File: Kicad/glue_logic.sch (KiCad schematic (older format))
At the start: 17 parts, among them U12 SN74LS273, U13 DM74AS74M, U14 DM74AS74M, U15 74AS04, U16 DM74S05M, U17 74F151A, U18 DM74AS74M, U19 74F151A, U37 DM74AS74M, U5 DM74S05M, U51 DM74AS74M, U7 DM74AS74M

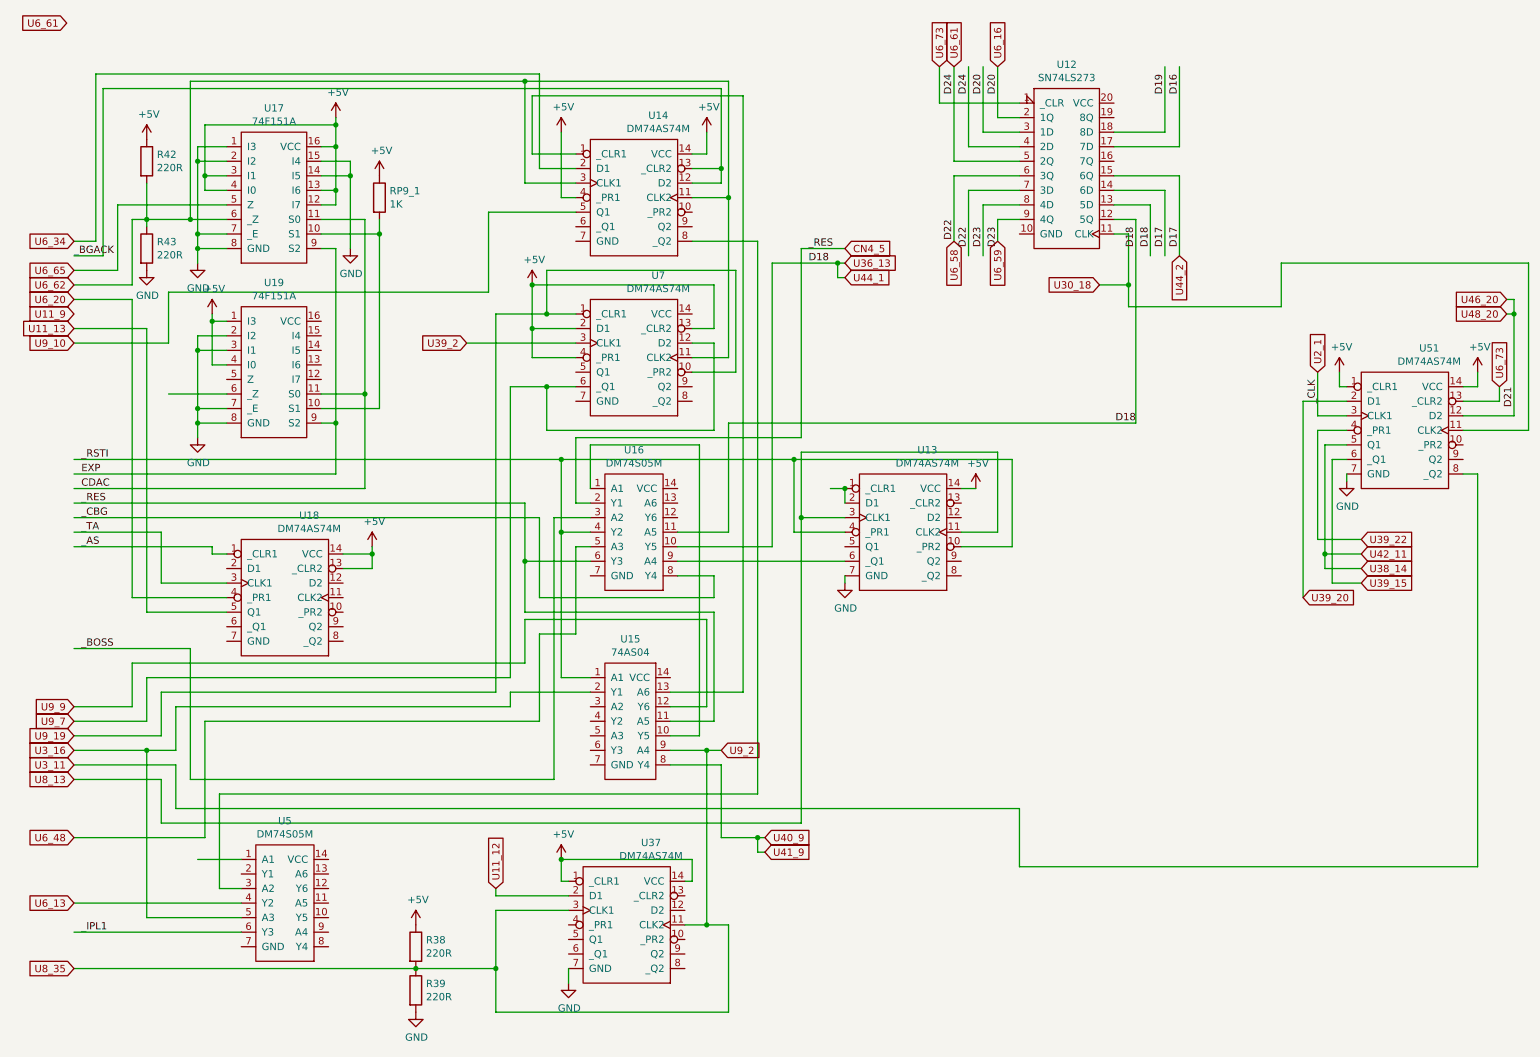
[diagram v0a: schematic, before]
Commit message: amother day, another tracks..
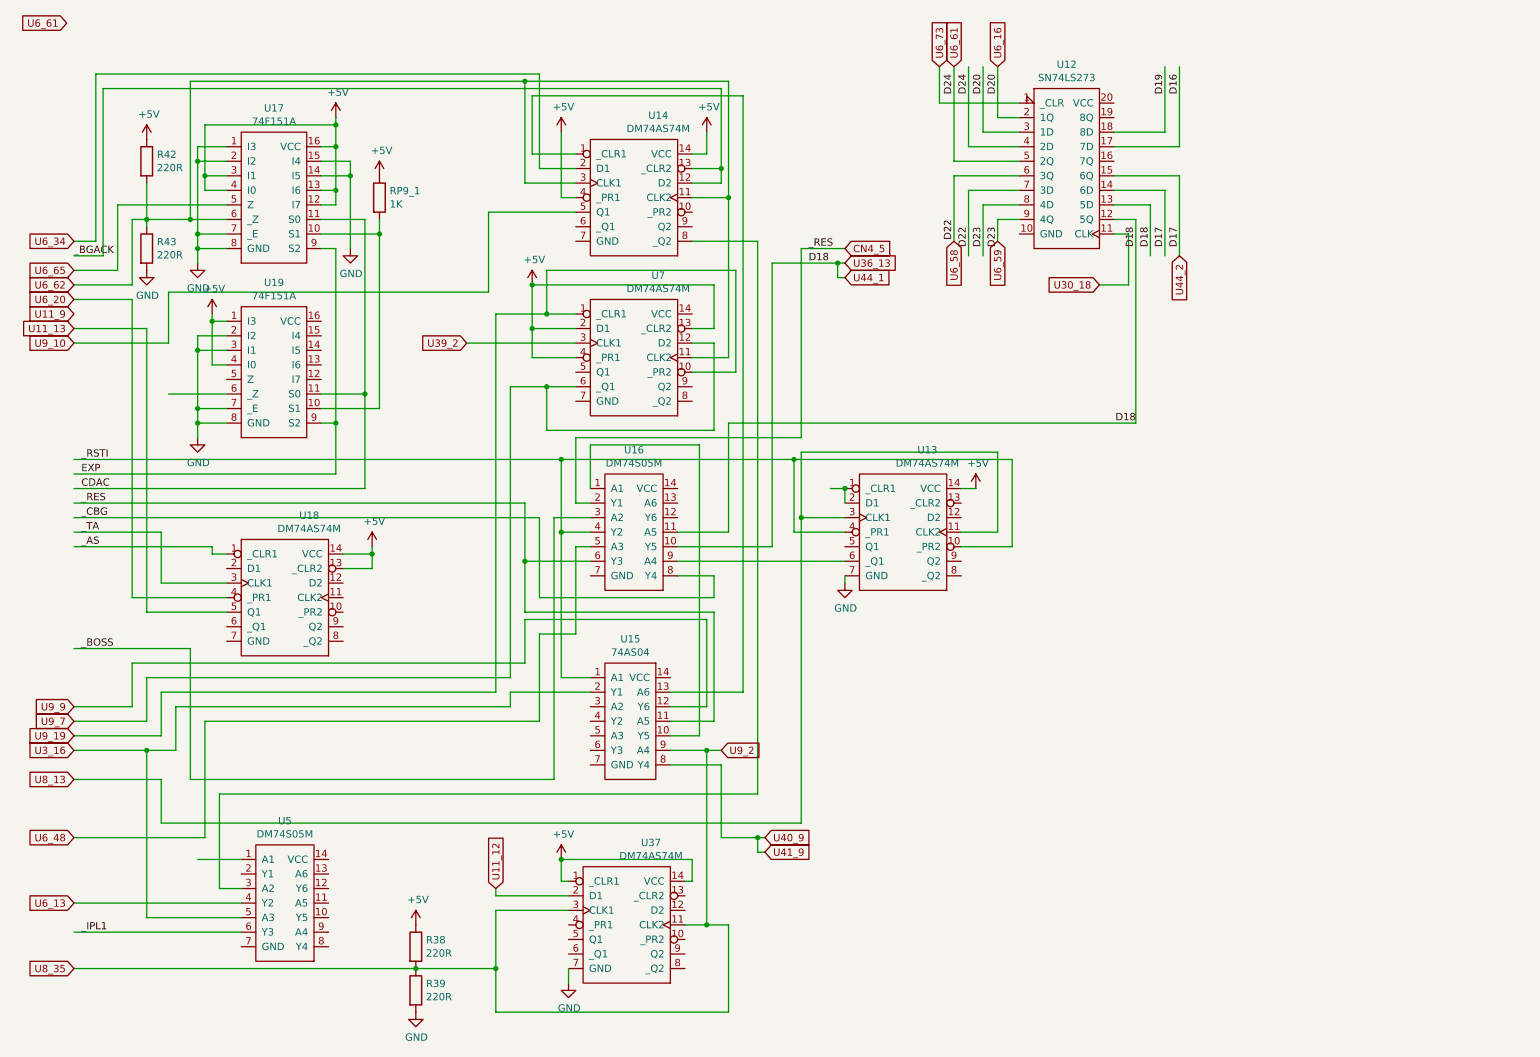
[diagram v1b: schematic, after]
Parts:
- removed U51: DM74AS74M, symbol New_Library_0:DM74AS74M
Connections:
- net labels removed: D21, U2_1, U38_14, U39_15, U39_20, U39_22, U3_11, U42_11, U46_20, U48_20, _CLK
- wire segments 329 -> 289
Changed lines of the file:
@@
 Wire Wire Line
 	4100 5250 4650 5250
-Text GLabel 1100 5750 0    50   Input ~ 0
-U3_11
-Wire Wire Line
-	1800 6050 1800 5750
-Wire Wire Line
-	1800 5750 1100 5750
 Text GLabel 1100 5850 0    50   Input ~ 0
 U8_13
@@
 Wire Wire Line
 	2250 6700 1100 6700
-Wire Wire Line
-	2100 5950 2100 6600
-Wire Wire Line
-	2100 6600 2250 6600
-Wire Wire Line
-	2100 5950 5800 5950
 Wire Wire Line
 	5800 5950 5800 2150
@@
 Wire Wire Line
 	3150 4300 3150 4250
-Wire Wire Line
-	10750 3150 10650 3150
-Wire Wire Line
-	10750 3050 10750 3150
-$Comp
-L power:+5V #PWR?
-U 1 1 5DC2CB2C
-P 10750 3050
-F 0 "#PWR?" H 10750 2900 50  0001 C CNN
-F 1 "+5V" H 10765 3223 50  0000 C CNN
-F 2 "" H 10750 3050 50  0001 C CNN
-F 3 "" H 10750 3050 50  0001 C CNN
-	1    10750 3050
-	1    0    0    -1
-$EndComp
-Wire Wire Line
-	9850 3800 9850 3750
-$Comp
-L power:GND #PWR?
-U 1 1 5DC0BA94
-P 9850 3800
-F 0 "#PWR?" H 9850 3550 50  0001 C CNN
-F 1 "GND" H 9855 3627 50  0000 C CNN
-F 2 "" H 9850 3800 50  0001 C CNN
-F 3 "" H 9850 3800 50  0001 C CNN
-	1    9850 3800
-	1    0    0    -1
-$EndComp
-Text GLabel 9550 4600 2    50   Input ~ 0
-U39_20
-Wire Wire Line
-	9850 3250 9550 3250
-Wire Wire Line
-	9750 4500 9950 4500
-Wire Wire Line
-	9750 3650 9750 4500
-Wire Wire Line
-	9850 3650 9750 3650
-Text GLabel 9950 4500 2    50   Input ~ 0
-U39_15
-Connection ~ 9700 4300
-Wire Wire Line
-	9700 4400 9700 4300
-Wire Wire Line
-	9950 4400 9700 4400
-Wire Wire Line
-	9700 4300 9950 4300
-Wire Wire Line
-	9700 3550 9700 4300
-Wire Wire Line
-	9850 3550 9700 3550
-Text GLabel 9950 4400 2    50   Input ~ 0
-U38_14
-Text GLabel 9950 4300 2    50   Input ~ 0
-U42_11
-Wire Wire Line
-	9650 4200 9950 4200
-Wire Wire Line
-	9650 3450 9650 4200
-Wire Wire Line
-	9850 3450 9650 3450
-Text GLabel 9950 4200 2    50   Input ~ 0
-U39_22
 Text GLabel 5850 6350 2    50   Input ~ 0
 U41_9
@@
 U40_9
 Wire Wire Line
-	9800 3150 9850 3150
-Wire Wire Line
-	9800 3050 9800 3150
-$Comp
-L power:+5V #PWR?
-U 1 1 5D8F16EA
-P 9800 3050
-F 0 "#PWR?" H 9800 2900 50  0001 C CNN
-F 1 "+5V" H 9815 3223 50  0000 C CNN
-F 2 "" H 9800 3050 50  0001 C CNN
-F 3 "" H 9800 3050 50  0001 C CNN
-	1    9800 3050
-	1    0    0    -1
-$EndComp
-$Comp
-L New_Library_0:DM74AS74M U51
-U 1 1 5DC69CD6
-P 10250 3450
-F 0 "U51" H 10417 4015 50  0000 C CNN
-F 1 "DM74AS74M" H 10417 3924 50  0000 C CNN
-F 2 "" H 10250 3450 50  0001 C CNN
-F 3 "" H 10250 3450 50  0001 C CNN
-	1    10250 3450
-	1    0    0    -1
-$EndComp
-Wire Wire Line
-	9550 3250 9550 4600
-Wire Wire Line
-	7600 6050 7600 6450
-Wire Wire Line
-	10750 6450 10750 3750
-Wire Wire Line
-	10750 3750 10650 3750
-Wire Wire Line
-	1800 6050 7600 6050
-Wire Wire Line
-	7600 6450 10750 6450
-Wire Wire Line
-	11100 2300 9400 2300
-Wire Wire Line
 	8350 2100 8350 2450
 Wire Wire Line
 	8150 2450 8350 2450
-Text GLabel 10900 3150 1    50   Input ~ 0
-U6_73
-Wire Wire Line
-	10900 3150 10900 3250
-Wire Wire Line
-	10650 3250 10900 3250
-Wire Wire Line
-	9850 3350 9650 3350
-Wire Wire Line
-	9650 3350 9650 3050
-Text GLabel 9650 3050 1    50   Input ~ 0
-U2_1
-Text Label 9650 3100 3    50   ~ 0
-_CLK
-Wire Wire Line
-	10650 3350 11000 3350
-Text Label 11000 3150 3    50   ~ 0
-D21
-Text GLabel 10950 2650 0    50   Input ~ 0
-U48_20
-Text GLabel 10950 2550 0    50   Input ~ 0
-U46_20
-Wire Wire Line
-	11000 2550 10950 2550
-Wire Wire Line
-	11000 2550 11000 2650
-Wire Wire Line
-	10950 2650 11000 2650
-Connection ~ 11000 2650
-Wire Wire Line
-	11000 2650 11000 3350
 Wire Wire Line
 	8250 2000 8400 2000
@@
 Text Label 8400 3400 2    50   ~ 0
 D18
-Wire Wire Line
-	11100 3450 11100 2300
-Wire Wire Line
-	10650 3450 11100 3450
-Wire Wire Line
-	8350 2450 8350 2600
-Wire Wire Line
-	8350 2600 9400 2600
-Wire Wire Line
-	9400 2600 9400 2300
-Connection ~ 8350 2450
 Wire Wire Line
 	8400 2000 8400 3400
@@
 Text Label 6150 2300 0    50   ~ 0
 D18
+Wire Wire Line
+	2100 5950 5800 5950
+Wire Wire Line
+	2100 6600 2250 6600
+Wire Wire Line
+	2100 5950 2100 6600
 $EndSCHEMATC
